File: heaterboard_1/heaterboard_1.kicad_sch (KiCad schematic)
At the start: 52 parts, among them J1 Barrel_Jack_Switch_SMT, J10 Conn_02x05_Odd_Even, J11 Screw_Terminal_01x02, J2 HS96L03W2C03_0.96_Oled, J5 Conn_02x05_Odd_Even, J6 Screw_Terminal_01x06, J9 Screw_Terminal_01x06, Q1 IRF540N, Q2 BSS138, SW1 6mm 2 Pin Tact NO Breadboard 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, SW2 6mm 2 Pin Tact NO Breadboard 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, SW3 6mm 2 Pin Tact NO Breadboard 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, U1 TMP36GRTZ-REEL7

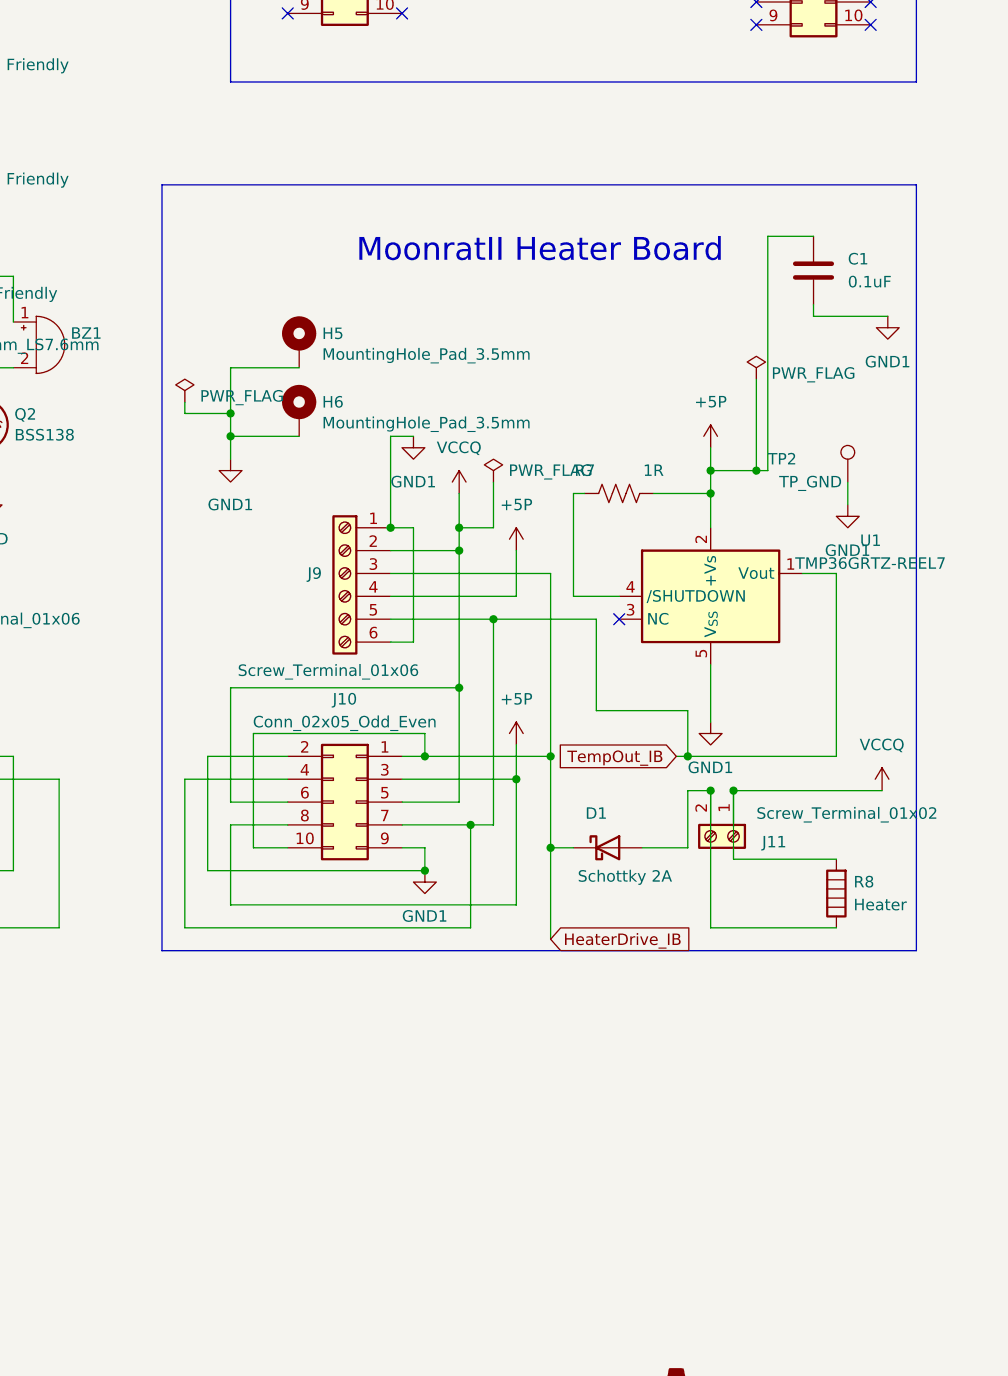
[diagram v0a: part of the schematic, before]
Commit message: heaterboard_1.kicad_sch Replacing TMP36 with TSIC206-TO92.
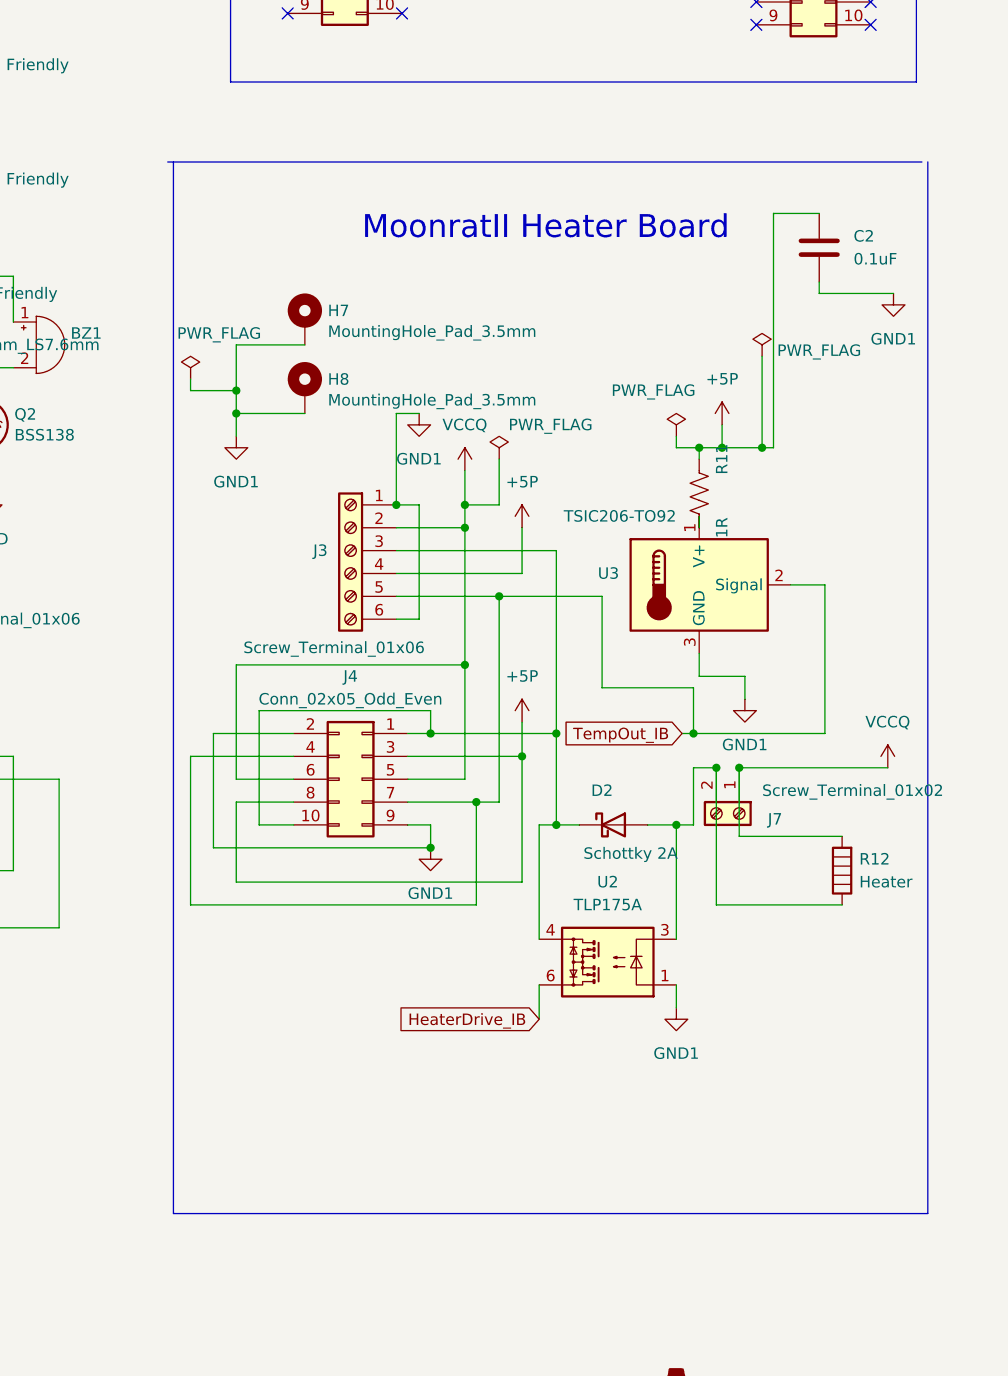
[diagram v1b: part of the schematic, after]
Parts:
- removed C1: 0.1uF, Capacitor_SMD:C_0603_1608Metric_Pad1.08x0.95mm_HandSolder, symbol Device:C
- removed D1: Schottky 2A, Diode_SMD:D_SMB, symbol Device:D_Schottky
- removed H5, H6: MountingHole_Pad_3.5mm, GeneralPurposeAlarmDevicePCB:MountingHole_3.5mm_Pad_Via, symbol GPAD_SCH_LIB:MountingHole_Pad_3.5mm
- removed J10: Conn_02x05_Odd_Even, Connector_IDC:IDC-Header_2x05_P2.54mm_Vertical, symbol Connector_Generic:Conn_02x05_Odd_Even
- removed J11: Screw_Terminal_01x02, TerminalBlock_TE-Connectivity:TerminalBlock_TE_282834-2_1x02_P2.54mm_Horizontal, symbol Connector:Screw_Terminal_01x02
- removed J9: Screw_Terminal_01x06, GeneralPurposeAlarmDevicePCB:1x6P 20A -40℃~+105℃ 300V Green 12~30 Straight pin 5.08mm 2.5 1 6 Plugin,P=5.08mm Screw ter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, symbol Connector:Screw_Terminal_01x06
- removed R7: 1R, Resistor_SMD:R_0603_1608Metric_Pad0.98x0.95mm_HandSolder, symbol Device:R_US
- removed R8: Heater, symbol Device:Heater
- removed TP2: TP_GND, TestPoint:TestPoint_Loop_D2.54mm_Drill1.5mm_Beaded, symbol Connector:TestPoint
- removed U1: TMP36GRTZ-REEL7, Package_TO_SOT_SMD:SOT-23-5, symbol GPAD_SCH_LIB:TMP36GRTZ-REEL7
- added C2: 0.1uF, Capacitor_SMD:C_0603_1608Metric_Pad1.08x0.95mm_HandSolder, symbol Device:C
- added D2: Schottky 2A, Diode_SMD:D_SMB, symbol Device:D_Schottky
- added H7, H8: MountingHole_Pad_3.5mm, GeneralPurposeAlarmDevicePCB:MountingHole_3.5mm_Pad_Via, symbol GPAD_SCH_LIB:MountingHole_Pad_3.5mm
- added J3: Screw_Terminal_01x06, GeneralPurposeAlarmDevicePCB:1x6P 20A -40℃~+105℃ 300V Green 12~30 Straight pin 5.08mm 2.5 1 6 Plugin,P=5.08mm Screw ter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, symbol Connector:Screw_Terminal_01x06
- added J4: Conn_02x05_Odd_Even, Connector_IDC:IDC-Header_2x05_P2.54mm_Vertical, symbol Connector_Generic:Conn_02x05_Odd_Even
- added J7: Screw_Terminal_01x02, TerminalBlock_TE-Connectivity:TerminalBlock_TE_282834-2_1x02_P2.54mm_Horizontal, symbol Connector:Screw_Terminal_01x02
- added R11: 1R, Resistor_SMD:R_0603_1608Metric_Pad0.98x0.95mm_HandSolder, symbol Device:R_US
- added R12: Heater, symbol Device:Heater
- added U2: TLP175A, Package_SO:MFSOP6-4_4.4x3.6mm_P1.27mm, symbol Relay_SolidState:TLP175A
- added U3: TSIC206-TO92, Package_TO_SOT_THT:TO-92_Inline, symbol Sensor_Temperature:TSIC206-TO92
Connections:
- net +5P: now also C2.1, J3.4 (Pin_4), J4.3 (Pin_3), J4.8 (Pin_8), R11.1
- net GND1: now also C2.2, H7.1, H8.1, J3.1 (Pin_1), J3.6 (Pin_6), J4.2 (Pin_2), J4.9 (Pin_9), U2.1, U3.3 (GND)
- net HeaterDrive_IB: now also U2.6
- net TempOut_IB: now also J3.5 (Pin_5), J4.4 (Pin_4), J4.7 (Pin_7), U3.2 (Signal)
- net VCCQ: now also J3.2 (Pin_2), J4.5 (Pin_5), J4.6 (Pin_6), J7.1 (Pin_1), R12.2
- new net: D2.1 (K), J3.3 (Pin_3), J4.1 (Pin_1), J4.10 (Pin_10), U2.4
- new net: R11.2, U3.1 (V+)
- new net: D2.2 (A), J7.2 (Pin_2), R12.1, U2.3
- no-connect marks 48 -> 47
